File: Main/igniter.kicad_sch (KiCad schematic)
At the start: 28 parts, among them IC7 PS2801C-4-F3-A, J7 Screw_Terminal_01x06, J8 JSTXH-1x02, Q2 BSS138, Q3 BSS138, Q4 BSS138, U1 Opamp_Quad

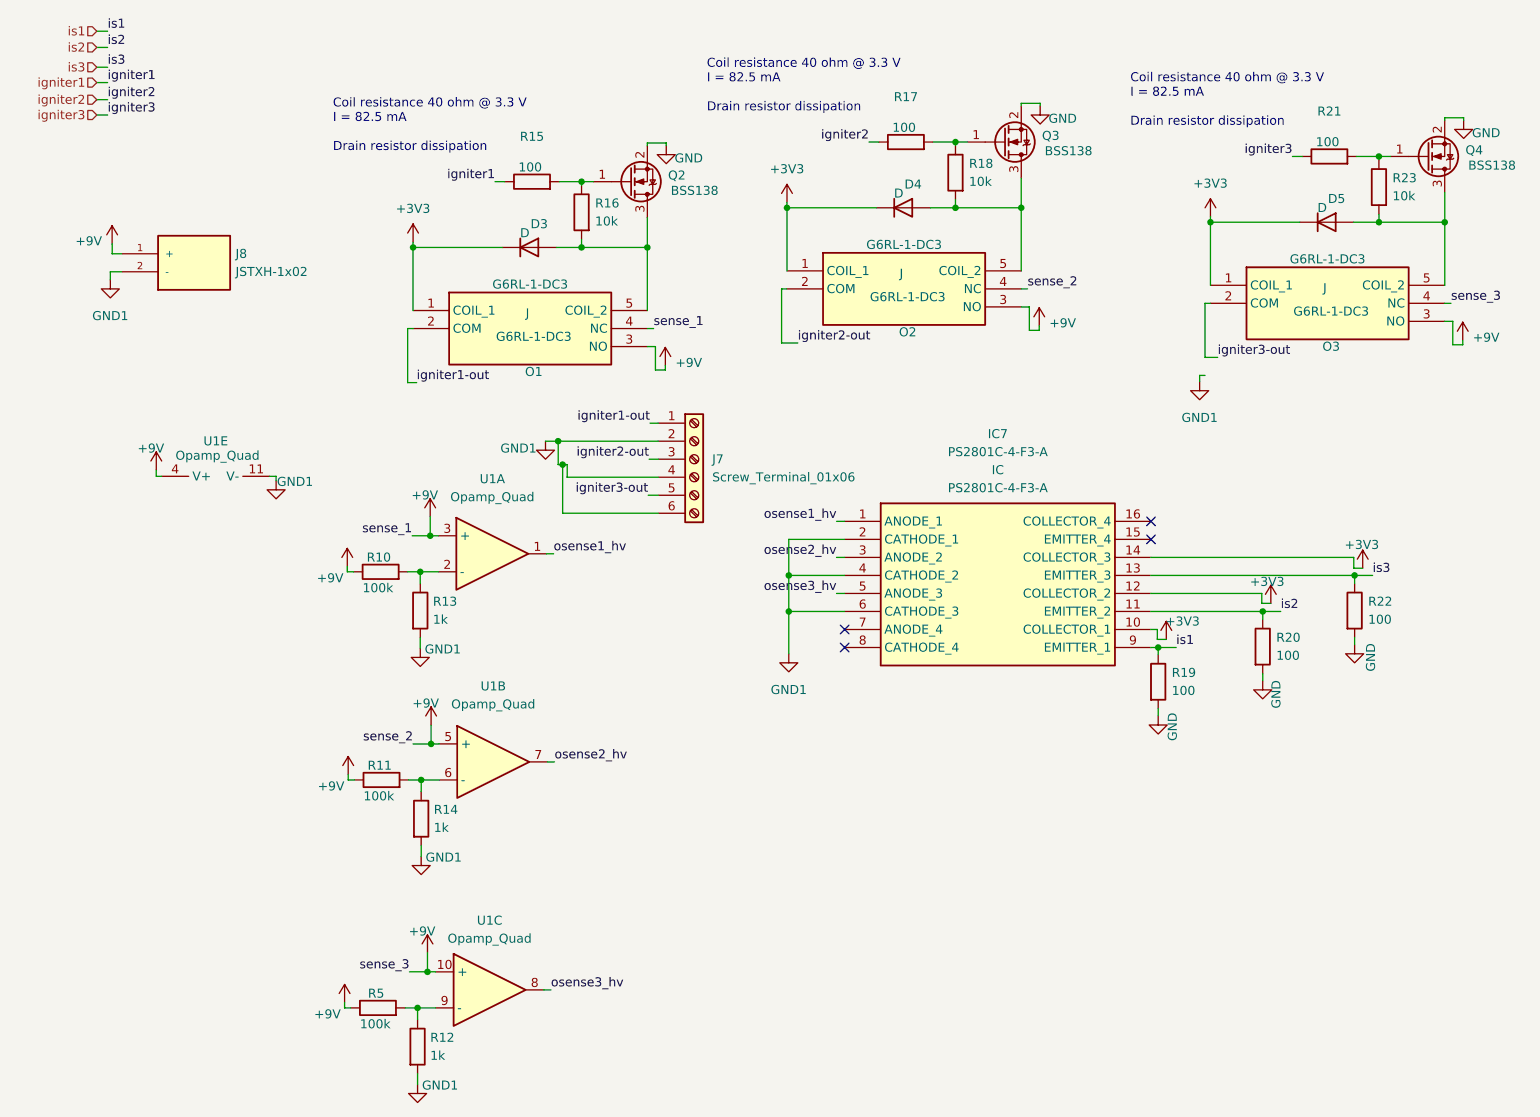
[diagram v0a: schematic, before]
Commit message: finalized pcb
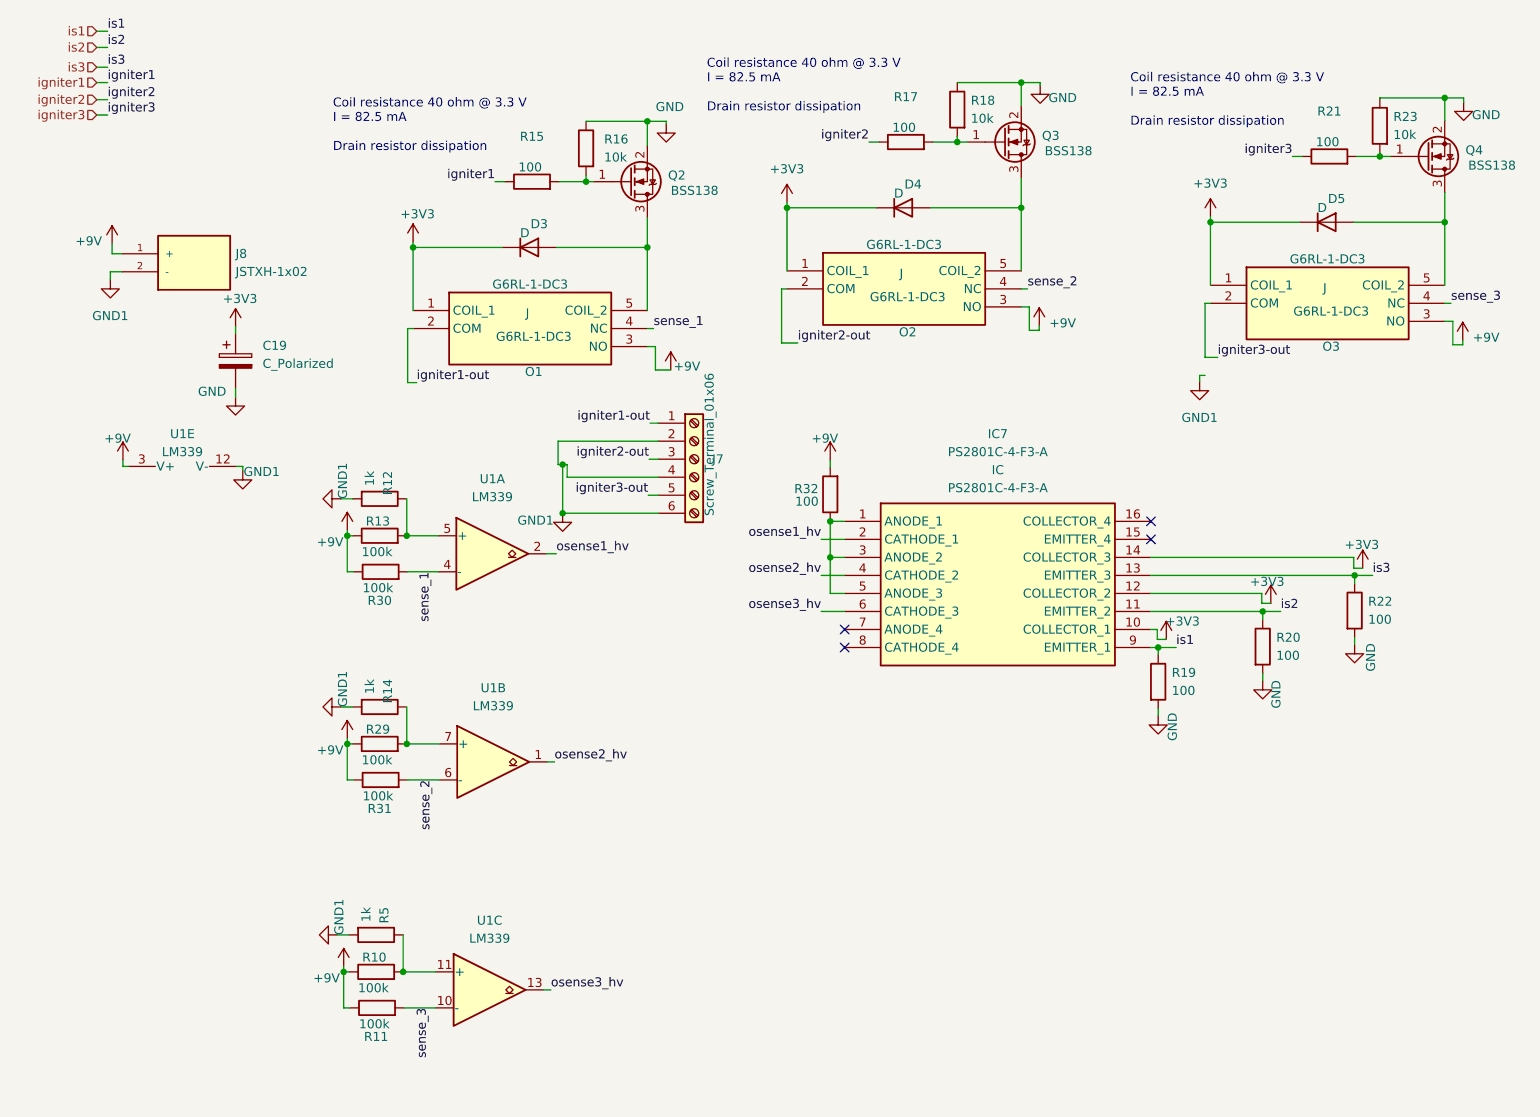
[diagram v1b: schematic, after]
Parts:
- removed U1: Opamp_Quad, Attiny414:SOIC127P600X175-14N, symbol Device:Opamp_Quad
- added C19: C_Polarized, Capacitor_SMD:CP_Elec_6.3x7.7, symbol Device:C_Polarized
- added R29, R30, R31: 100k, Resistor_SMD:R_0603_1608Metric, symbol Device:R
- added R32: 100, Resistor_SMD:R_0603_1608Metric, symbol Device:R
- added U1: LM339, Package_SO:TSSOP-14_4.4x5mm_P0.65mm, symbol Comparator:LM339
- R13: value 1k -> 100k
- R5: value 100k -> 1k
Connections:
- net +3V3: now also C19.1
- net +9V: now also R13.1, R29.1, R30.1, R31.1, R32.2, U1.3 (V+); no longer O1.4 (NC), O2.4 (NC), O3.4 (NC), R5.1
- net GND: now also R16.1, R18.1, R23.1, C19.2
- net GND1: now also R5.2, U1.12 (V-); no longer IC7.2 (CATHODE_1), IC7.4 (CATHODE_2), IC7.6 (CATHODE_3), R13.2
- net osense1_hv: now also IC7.2 (CATHODE_1), U1.2; no longer IC7.1 (ANODE_1)
- net osense2_hv: now also IC7.4 (CATHODE_2), U1.1; no longer IC7.3 (ANODE_2)
- net osense3_hv: now also IC7.6 (CATHODE_3), U1.13; no longer IC7.5 (ANODE_3)
- net at Q2.1 (G), R15.2: now also R16.2; no longer R16.1
- net at D3.2 (A), O1.5 (COIL_2), Q2.3 (D): no longer R16.2
- net at Q3.1 (G), R17.2: now also R18.2; no longer R18.1
- net at D5.2 (A), O3.5 (COIL_2), Q4.3 (D): no longer R23.2
- net at Q4.1 (G), R21.2: now also R23.2; no longer R23.1
- net at R12.1: now also R13.2, U1.5 (+); no longer R5.2
- net at D4.2 (A), O2.5 (COIL_2), Q3.3 (D): no longer R18.2
- net at R14.1: now also R29.2, U1.7 (+); no longer R11.2
- net at R10.2: now also R5.1, U1.11 (+); no longer R13.1
- new net: IC7.1 (ANODE_1), IC7.3 (ANODE_2), IC7.5 (ANODE_3), R32.1
- new net sense_1: O1.4 (NC), R30.2, U1.4 (-)
- new net sense_2: O2.4 (NC), R31.2, U1.6 (-)
- new net sense_3: O3.4 (NC), R11.2, U1.10 (-)
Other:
- moved on the sheet: R16, R18, R23
